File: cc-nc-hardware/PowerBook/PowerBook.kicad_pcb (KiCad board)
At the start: 2 copper layers, 82.1 x 56.3 mm, 95 parts, among them J1 Conn_01x03_Male, J2 PB_SCSI_HD_Pins, J4 SW, SW1 SW_MEC_5E, U1 SN74CBTD3384, U2 SN74CBTD3384, U3 AMS1117-2.85, U4 LVT245, U5 LVT125, U6 LVT125, U7 LVT125, U8 74HC14, U9 LVT245

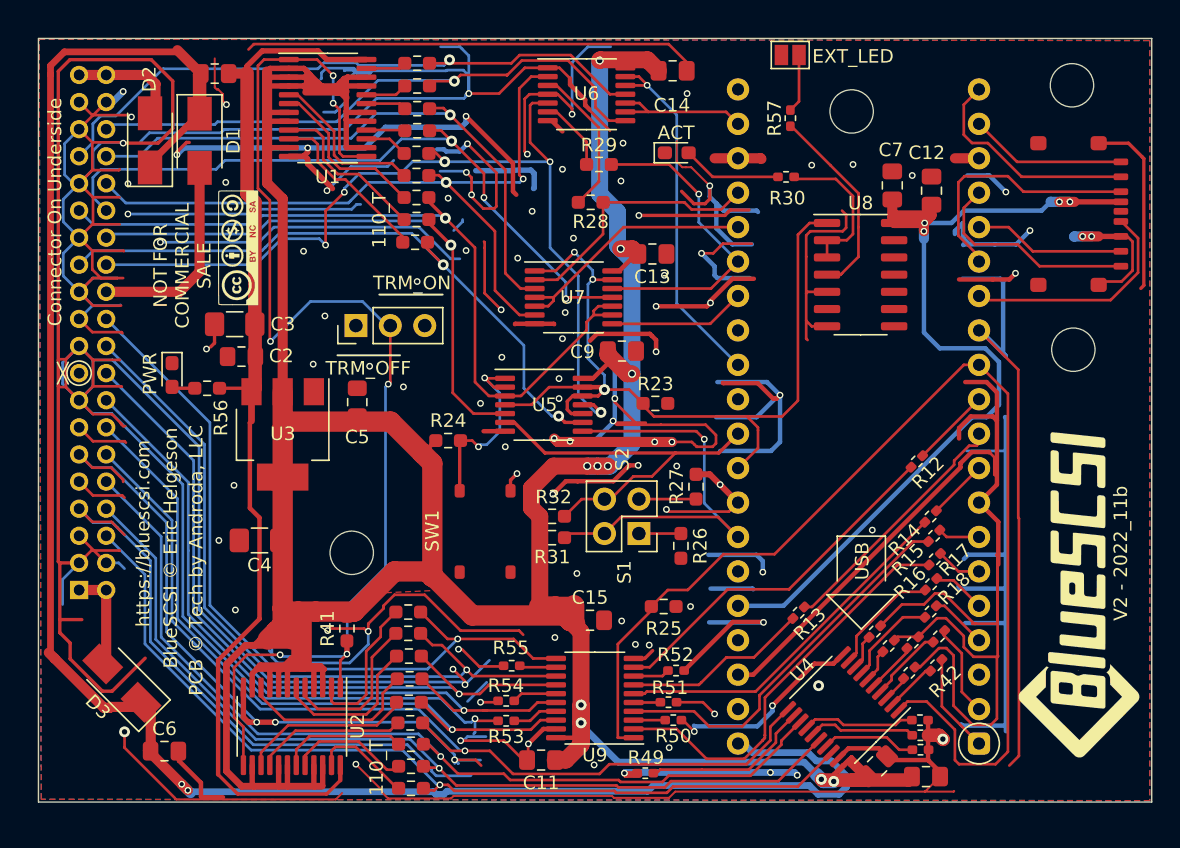
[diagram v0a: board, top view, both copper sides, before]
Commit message: PowerBook Hardware Version 2023.10a
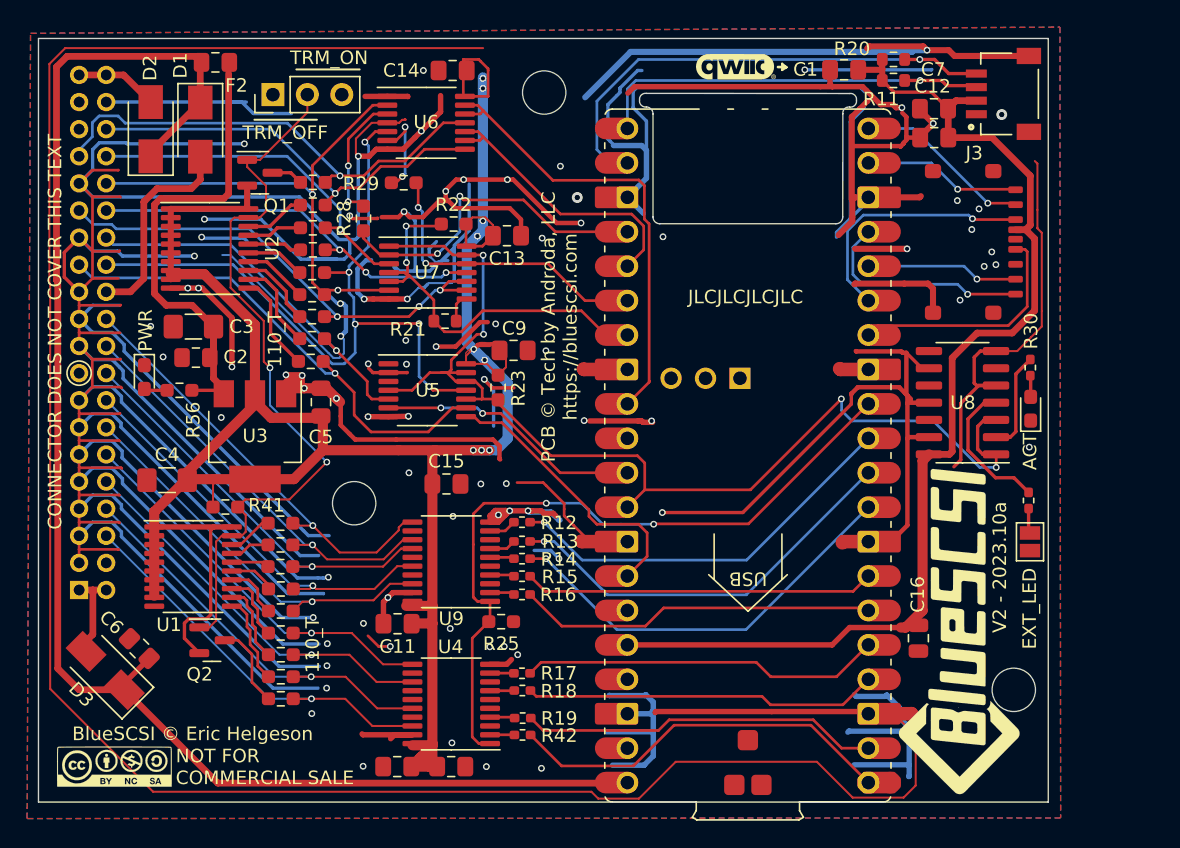
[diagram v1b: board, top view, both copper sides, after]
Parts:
- removed H4: MountingHole, MountingHole:MountingHole_3.2mm_M3
- removed J4: SW, Connector_PinHeader_2.54mm:PinHeader_2x02_P2.54mm_Vertical
- removed R24, R26, R27: 1k, Resistor_SMD:R_0603_1608Metric_Pad0.98x0.95mm_HandSolder
- removed R31, R32: 4.7k, Resistor_SMD:R_0603_1608Metric_Pad0.98x0.95mm_HandSolder
- removed R43, R44, R45, R46, R47, R48, R49, R50, R51, R52, R53, R54, R55: 1k, Resistor_SMD:R_0402_1005Metric_Pad0.72x0.64mm_HandSolder
- removed SW1: SW_MEC_5E, Library:TS-1187A-B-A-B
- added C1: 0.1uF, Capacitor_SMD:C_0805_2012Metric_Pad1.18x1.45mm_HandSolder, F.Cu at (159.5, 74.4)
- added C16: 0.1uF, Capacitor_SMD:C_0805_2012Metric, F.Cu at (165.0, 116.3)
- added G***: LOGO, LOGO, F.Cu at (151.5, 74.1)
- added J3: SM04B-SRSS-TB(LF)(SN), Library:JST_SM04B-SRSS-TB(LF)(SN), F.Cu at (169.3, 76.2)
- added Q1: AO3401A, Package_TO_SOT_SMD:SOT-23, F.Cu at (116.4, 82.0)
- added Q2: AO3401A, Package_TO_SOT_SMD:SOT-23, F.Cu at (112.9, 116.5)
- added R20: 4.7k, Resistor_SMD:R_0603_1608Metric, F.Cu at (163.2, 73.6)
- added R21: 1k, Resistor_SMD:R_0603_1608Metric, F.Cu at (130.1, 92.9)
- added R22: 1k, Resistor_SMD:R_0603_1608Metric_Pad0.98x0.95mm_HandSolder, F.Cu at (130.7, 85.8)
- R1, R10, R2, R3, R33, R34, R35, R36, R37, R38, R39, R4, R40, R5, R6, R7, R8, R9: value R -> 110
- R11: value 1k -> 4.7k; footprint Resistor_SMD:R_0402_1005Metric_Pad0.72x0.64mm_HandSolder -> Resistor_SMD:R_0603_1608Metric
- RP1: footprint CustomFootprints:BluePillModule -> Library:Raspberry_Pi_PicoW_SMT_THT
- U1, U2: value SN74CBTD3384 -> LVT245; footprint Package_SO:TSSOP-24_4.4x7.8mm_P0.65mm -> Package_SO:TSSOP-20_4.4x6.5mm_P0.65mm
- moved R11 43.7 mm to (163.2, 75.2), turned to 180 degrees
- moved JP1 40.0 mm to (173.2, 109.2), turned to -90 degrees
- moved G*** 39.4 mm to (105.7, 125.8), turned to 0 degrees
- moved H5 38.9 mm to (137.4, 76.1)
- moved U2 35.8 mm to (112.7, 87.6), turned to 0 degrees
- moved C8 35.4 mm to (126.5, 125.8), turned to 180 degrees
- moved U1 35.3 mm to (111.5, 111.0)
- moved C10 35.0 mm to (130.5, 125.8)
- moved R57 33.2 mm to (173.1, 106.2), turned to -90 degrees
- moved D4 32.2 mm to (173.3, 99.4), turned to 90 degrees
- moved R19 31.3 mm to (135.8, 122.2), turned to 180 degrees
- moved R42 30.9 mm to (135.8, 123.5), turned to 180 degrees
- moved R17 30.9 mm to (135.8, 118.9), turned to 180 degrees
- moved R18 30.7 mm to (135.8, 120.2), turned to 180 degrees
- moved R16 30.6 mm to (135.8, 113.1), turned to 180 degrees
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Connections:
- R11 pad 1: GND -> SDA
- R11 pad 2: Net-(R11-Pad2) -> +3V3
- R23 pad 2: GND -> +2V8
- R36 pad 1: Net-(R36-Pad1) -> Net-(Q2-Pad3)
- R6 pad 1: Net-(R6-Pad1) -> Net-(Q1-Pad3)
- RP1 pad 21: SERIAL_OUT -> SDA
- RP1 pad 22: oREQ -> SCL
- RP1 pad 25: oSEL -> oREQ
- RP1 pad 27: iRST -> oSEL
- U1 pad 1: TRM_ON_J -> +2V8
- U1 pad 10: Net-(R2-Pad1) -> GND
- U1 pad 11: +2V8 -> Net-(R37-Pad1)
- U1 pad 12: GND -> Net-(R38-Pad1)
- U1 pad 13: TRM_ON_J -> Net-(R39-Pad1)
- U1 pad 14: +2V8 -> Net-(R40-Pad1)
- U1 pad 15: Net-(R10-Pad1) -> Net-(R1-Pad1)
- U1 pad 16: Net-(R9-Pad1) -> Net-(R33-Pad1)
- U1 pad 17: +2V8 -> Net-(R34-Pad1)
- U1 pad 18: +2V8 -> Net-(R35-Pad1)
- U1 pad 19: Net-(R8-Pad1) -> TRM_ON_J
- U1 pad 20: Net-(R7-Pad1) -> +2V8
- U1 pad 5: Net-(R5-Pad1) -> +2V8
- U1 pad 6: Net-(R4-Pad1) -> +2V8
- U1 pad 9: Net-(R3-Pad1) -> +2V8
- U2 pad 1: TRM_ON_J -> +2V8
- U2 pad 10: Net-(R1-Pad1) -> GND
- U2 pad 11: +2V8 -> Net-(R2-Pad1)
- U2 pad 12: GND -> Net-(R3-Pad1)
- U2 pad 13: TRM_ON_J -> Net-(R4-Pad1)
- U2 pad 14: +2V8 -> Net-(R5-Pad1)
- U2 pad 15: Net-(R40-Pad1) -> Net-(R10-Pad1)
- U2 pad 16: Net-(R39-Pad1) -> Net-(R9-Pad1)
- U2 pad 17: +2V8 -> Net-(R8-Pad1)
- U2 pad 18: +2V8 -> Net-(R7-Pad1)
- U2 pad 19: Net-(R38-Pad1) -> TRM_ON_J
- U2 pad 2: Net-(R35-Pad1) -> +2V8
- U2 pad 20: Net-(R37-Pad1) -> +2V8
- U2 pad 5: Net-(R34-Pad1) -> +2V8
- U2 pad 6: Net-(R33-Pad1) -> +2V8
- U4 pad 12: Net-(R49-Pad1) -> unconnected-(U4-Pad12)
- U4 pad 14: Net-(R48-Pad1) -> unconnected-(U4-Pad14)
- U4 pad 15: Net-(R47-Pad1) -> unconnected-(U4-Pad15)
- U4 pad 17: Net-(R46-Pad1) -> unconnected-(U4-Pad17)
- U4 pad 3: Net-(R11-Pad2) -> unconnected-(U4-Pad3)
- U4 pad 5: Net-(R43-Pad2) -> unconnected-(U4-Pad5)
- U4 pad 6: Net-(R44-Pad2) -> unconnected-(U4-Pad6)
- U4 pad 8: Net-(R45-Pad2) -> unconnected-(U4-Pad8)
- U5 pad 1: oRST -> GND
- U5 pad 2: oRST -> GND
- U5 pad 3: RST -> unconnected-(U5-Pad3)
- U8 pad 3: Net-(R30-Pad1) -> oBSY
- U9 pad 12: Net-(R55-Pad1) -> unconnected-(U9-Pad12)
- U9 pad 15: Net-(R54-Pad1) -> unconnected-(U9-Pad15)
- U9 pad 17: Net-(R53-Pad1) -> unconnected-(U9-Pad17)
- U9 pad 3: Net-(R50-Pad2) -> unconnected-(U9-Pad3)
- U9 pad 5: Net-(R51-Pad2) -> unconnected-(U9-Pad5)
- U9 pad 8: Net-(R52-Pad2) -> unconnected-(U9-Pad8)
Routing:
- net GND: track 1180.6 -> 1017.9 mm, vias 106 -> 82
- net +2V8: track 333.4 -> 185.4 mm, vias 10 -> 9
- net +5F: track 79.9 -> 35.7 mm
- net DB3: track 71.0 -> 30.4 mm
- net DB2: track 68.4 -> 30.1 mm
- net DB1: track 67.2 -> 30.0 mm
- net DB0: track 67.0 -> 29.8 mm
- net SCL: track 0.00 -> 37.1 mm, vias 0 -> 1
- net TRM_ON_J: track 91.7 -> 55.1 mm, vias 6 -> 2
- net DBPTr: track 84.8 -> 53.4 mm, vias 0 -> 2
- net SDA: track 0.00 -> 30.3 mm, vias 0 -> 1
- net +5VP: track 141.0 -> 111.1 mm, vias 2 -> 0
- net DB4T: track 30.4 -> 1.82 mm
- net DB5T: track 28.4 -> 1.80 mm
- net Net-(R14-Pad1): track 4.45 -> 30.9 mm, vias 0 -> 1
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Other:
- board size 82.1 x 56.3 mm -> 74.5 x 56.3 mm
- board text added: "CONNECTOR DOES NOT COVER THIS TEXT"
- board text added: "JLCJLCJLCJLC"
- board text added: "PCB © Tech by Androda, LLC https://bluescsi.com"
- board text added: "V2 - 2023.10a"
- board text removed: "Connector On Underside"
- board text removed: "PCB © Tech by Androda, LLC"
- board text removed: "S1"
- board text removed: "S2"
- board text removed: "V2 - 2022_11b"
- board text removed: "https://bluescsi.com"
